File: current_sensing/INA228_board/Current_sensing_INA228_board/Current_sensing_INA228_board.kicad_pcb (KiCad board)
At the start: 2 copper layers, 42.8 x 36.2 mm, 26 parts, among them J1 7461096, J2 7461096, J3 Conn_01x06_Pin, U1 INA228

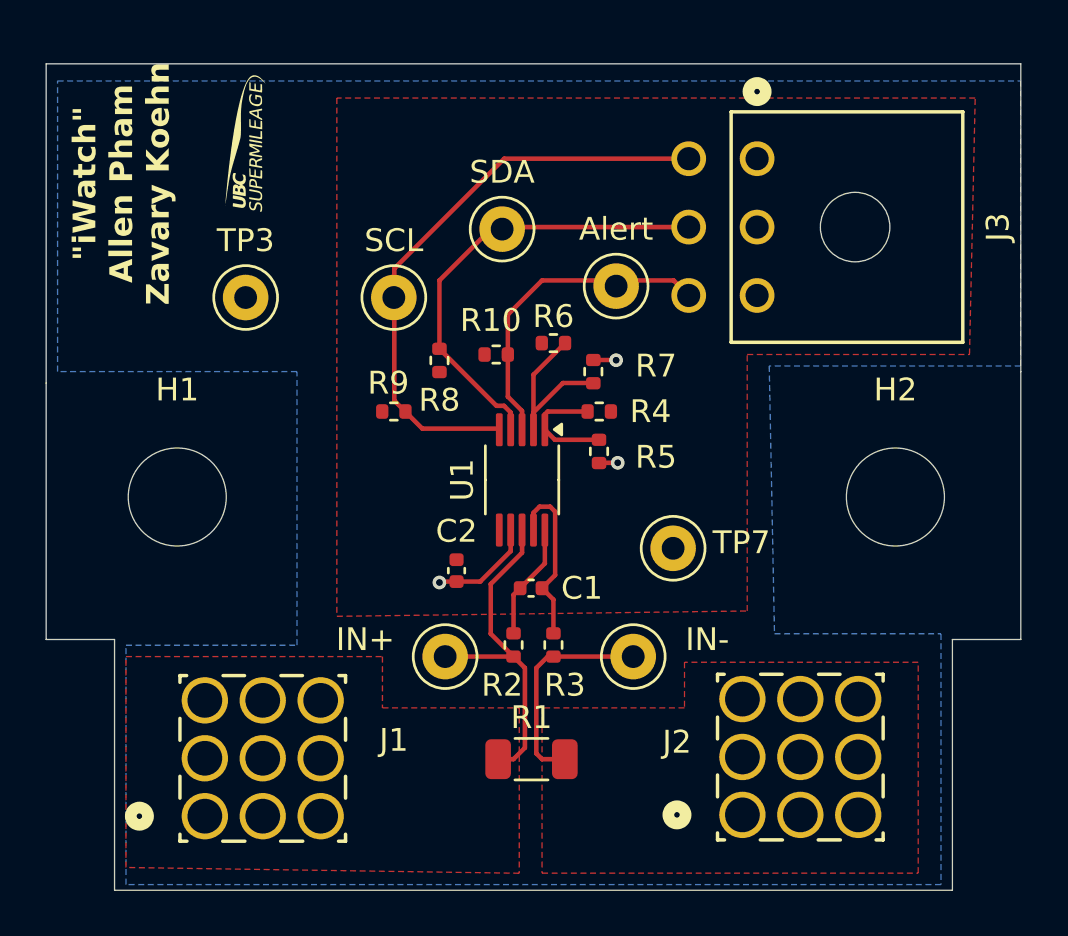
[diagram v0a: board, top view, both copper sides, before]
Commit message: Control Board schematics
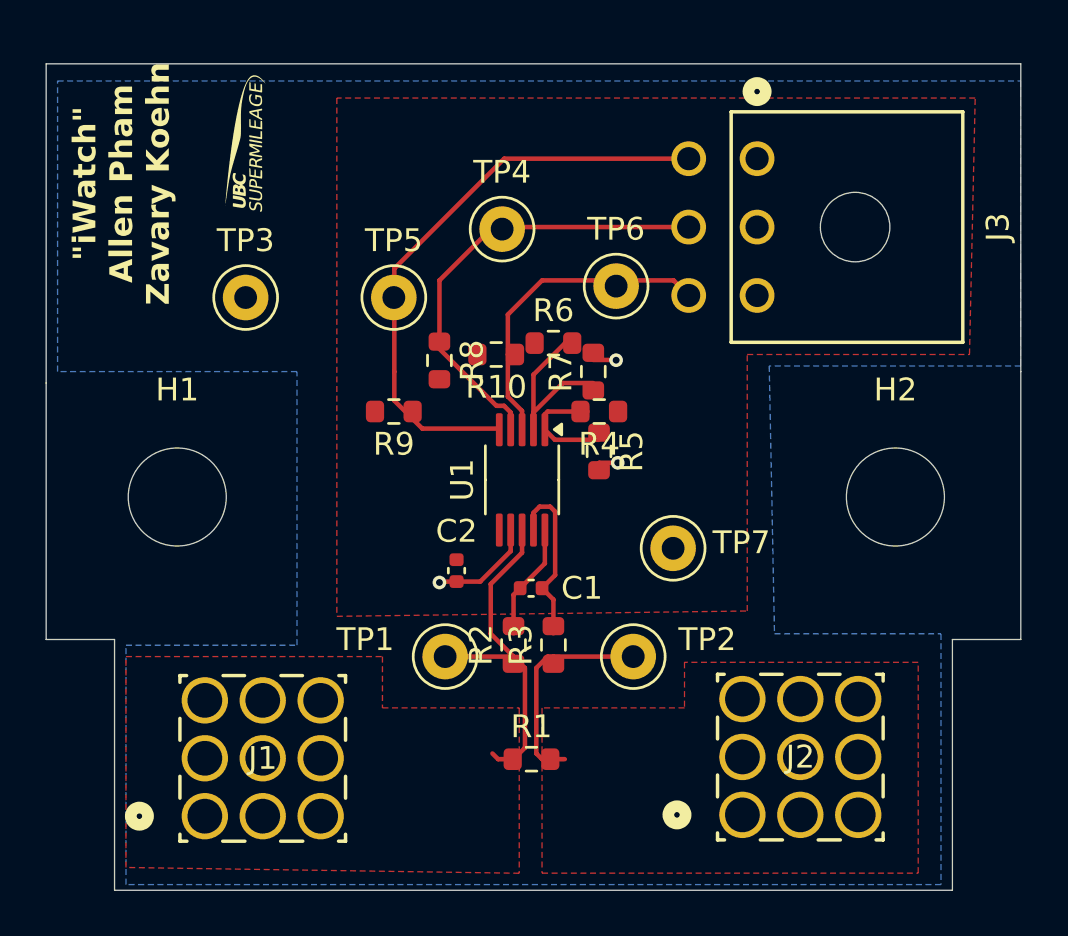
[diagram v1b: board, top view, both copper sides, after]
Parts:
- J1, J2: footprint ul_7461096:CONN9_1096_WRE -> footprints:CONN9_1096_WRE
- R1: footprint Resistor_SMD:R_1206_3216Metric -> Resistor_SMD:R_0603_1608Metric
- R10, R2, R3, R4, R5, R6, R7, R8, R9: footprint Resistor_SMD:R_0402_1005Metric -> Resistor_SMD:R_0603_1608Metric
- TP7: value 3.3V -> 5V
- renumbered IN+ to TP1, IN- to TP2, SDA to TP4, SCL to TP5, Alert to TP6
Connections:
- net +3.3V renamed +5V
